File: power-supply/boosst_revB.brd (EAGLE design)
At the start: 30.5 x 30.5 mm, 15 parts

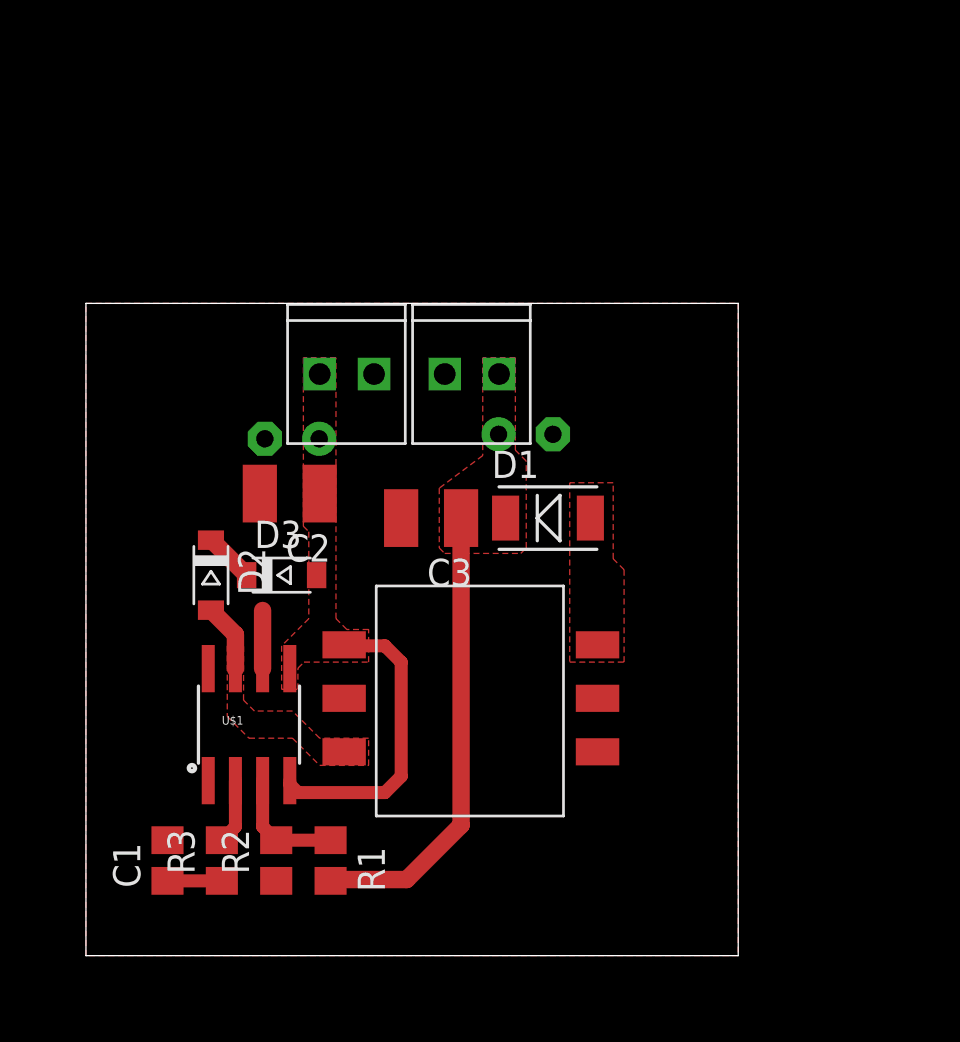
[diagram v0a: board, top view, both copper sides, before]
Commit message: slow progress
added new version for in4 PCB + some cleaning of files
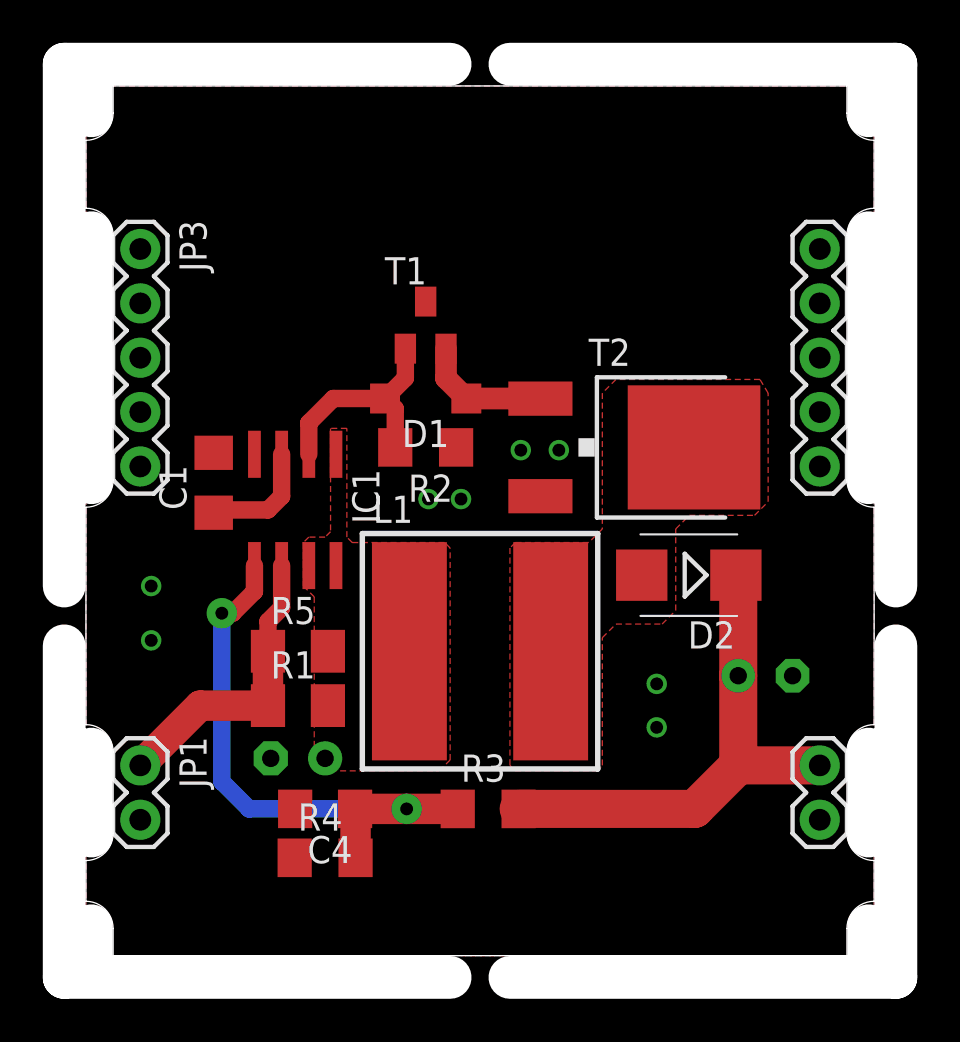
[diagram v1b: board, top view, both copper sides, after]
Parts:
- removed C5: (no value), rcl:E2,5-5
- removed D3: (no value), dp_devices:SOD-123
- removed U$1: MC3172YM, custom_lbr:SOIC8
- removed U$2: FA2469-ALB, custom_lbr:FA2469
- added IC1: MC34063AD, mc34063:SOIC8
- added JP3, JP4: (no value), SparkFun-Connectors:1X05
- added L1: SRN1060, custom_lbr:SRN1060
- added R4: (no value), rcl:R1206
- added R5: (no value), rcl:M1206
- added T1: (no value), transistor:SOT23-BEC
- added T2: IRFR220N, custom_lbr:DPACK
- C1: device rcl:C0805 -> rcl:C1206
- C2: device rcl:C1210 -> rcl:E2,5-6
- C3: device rcl:C1210 -> rcl:E2,5-6E
- C4: device rcl:E2,5-5 -> rcl:C1206
- D1: device dp_devices:DO-214AC -> diode:SOD123
- D2: device dp_devices:SOD-123 -> diode:SMB
- JP1, JP2: device SparkFun-Connectors:1X02_2.54_SCREWTERM -> SparkFun-Connectors:1X02
- R1: device rcl:R0805 -> rcl:M1206
- R2, R3: device rcl:R0805 -> rcl:R1206
- moved JP2 29.7 mm to (34.3, 8.89), turned to 270 degrees
- moved JP1 23.2 mm to (2.54, 8.89), turned to 270 degrees
- moved D2 22.3 mm to (28.2, 17.8), turned to 180 degrees
- moved R2 20.5 mm to (15.9, 23.7), turned to 180 degrees
- moved C1 17.8 mm to (5.97, 22.1)
- moved C4 17.4 mm to (11.2, 6.86), flipped to the top, turned to 180 degrees
- moved C3 17.3 mm to (31.8, 13.1), flipped to the bottom
- moved R3 12.7 mm to (18.8, 6.86), turned to 0 degrees
- moved C2 12.4 mm to (9.91, 9.22), flipped to the bottom, turned to 0 degrees
- moved D1 7.99 mm to (15.9, 26.0), turned to 180 degrees
- moved R1 7.40 mm to (9.91, 11.7), turned to 0 degrees
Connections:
- removed net N$8: C1.1, R3.1
- new net N$6: C2.+, IC1.1, IC1.7, IC1.8, L1.P$2, R1.2, R5.2
- net GND: now also C2.-, C3.-, C4.2, IC1.4, JP1.2, JP2.2, R4.1, T1.C, T2.3; no longer C2.2, C3.2, C4.-, C5.-, JP1.P2, JP2.P1, U$1.1, U$1.6, U$1.8, U$2.6
- net N$2: now also D1.C, T1.E, T2.1; no longer D2.C, D3.C
- net N$3: now also D1.A, IC1.2, R2.2, T1.B; no longer D1.2, U$2.4
- net N$4: now also C1.1, IC1.3; no longer R3.2, U$1.2
- net N$5: now also C4.1, IC1.5, R3.1, R4.2; no longer R1.1, R2.2, U$1.3
- net SW: now also L1.P$1, T2.4; no longer U$1.7, U$2.1
- net VIN: now also IC1.6, JP1.1, R1.1, R5.1; no longer C2.1, C4.+, D3.A, JP2.P2, U$1.4, U$1.5, U$2.3
- net VOUT: now also C3.+, D2.C, JP2.1, R3.2; no longer C3.1, C5.+, D1.1, JP1.P1, R1.2
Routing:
- net N$5: track 5.59 -> 27.3 mm, vias 0 -> 2
- net N$3: track 0.00 -> 10.7 mm
- net N$2: track 2.34 -> 7.11 mm
- net SW: track 3.21 -> 0.00 mm
- net GND: track 2.72 -> 0.00 mm, vias 0 -> 8
- net N$8: track 2.54 -> 0.00 mm
- net VOUT: track 21.5 -> 24.0 mm
- net N$4: track 3.05 -> 5.46 mm
- added copper zone on layer 16, net GND
- added copper zone on layer 1, net N$6
- removed copper zone on layer 1, net N$3
- removed copper zone on layer 1, net VIN
- removed copper zone on layer 1, net VOUT
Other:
- board size 30.5 x 30.5 mm -> 38.9 x 42.7 mm
